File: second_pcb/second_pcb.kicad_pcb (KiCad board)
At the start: 2 copper layers, 99.2 x 69.6 mm, 194 parts, among them SW1 SW_Nidec_CAS-120A1, U1 MIC29502WU, U10 CJ432, U11 CJ432, U12 CJ432, U13 CJ432, U14 CJ432, U15 CJ432, U16 CJ432, U17 CJ432, U18 CJ432, U19 CJ432, U2 CJ432, U20 CJ432, U21 CJ432, U22 CJ432, U23 CJ432, U24 CJ432, U25 CJ432, U26 CJ432, U27 CJ432, U28 CJ432, U29 CJ432, U3 CJ432, U30 CJ432, U31 CJ432, U32 CJ432, U33 CJ432, U34 CJ432, U35 CJ432, U36 CJ432, U37 CJ432, U38 CJ432, U39 CJ432, U4 CJ432, U40 CJ432, U41 CJ432, U42 CJ432, U43 CJ432, U44 CJ432, U45 CJ432, U46 CJ432, U47 CJ432, U48 CJ432, U49 CJ432, U5 CJ432, U50 CJ432, U51 CJ432, U52 CJ432, U53 CJ432, U54 CJ432, U55 CJ432, U56 CJ432, U57 CJ432, U58 CJ432, U59 CJ432, U6 CJ432, U60 CJ432, U61 CJ432, U7 CJ432, U8 CJ432, U9 CJ432

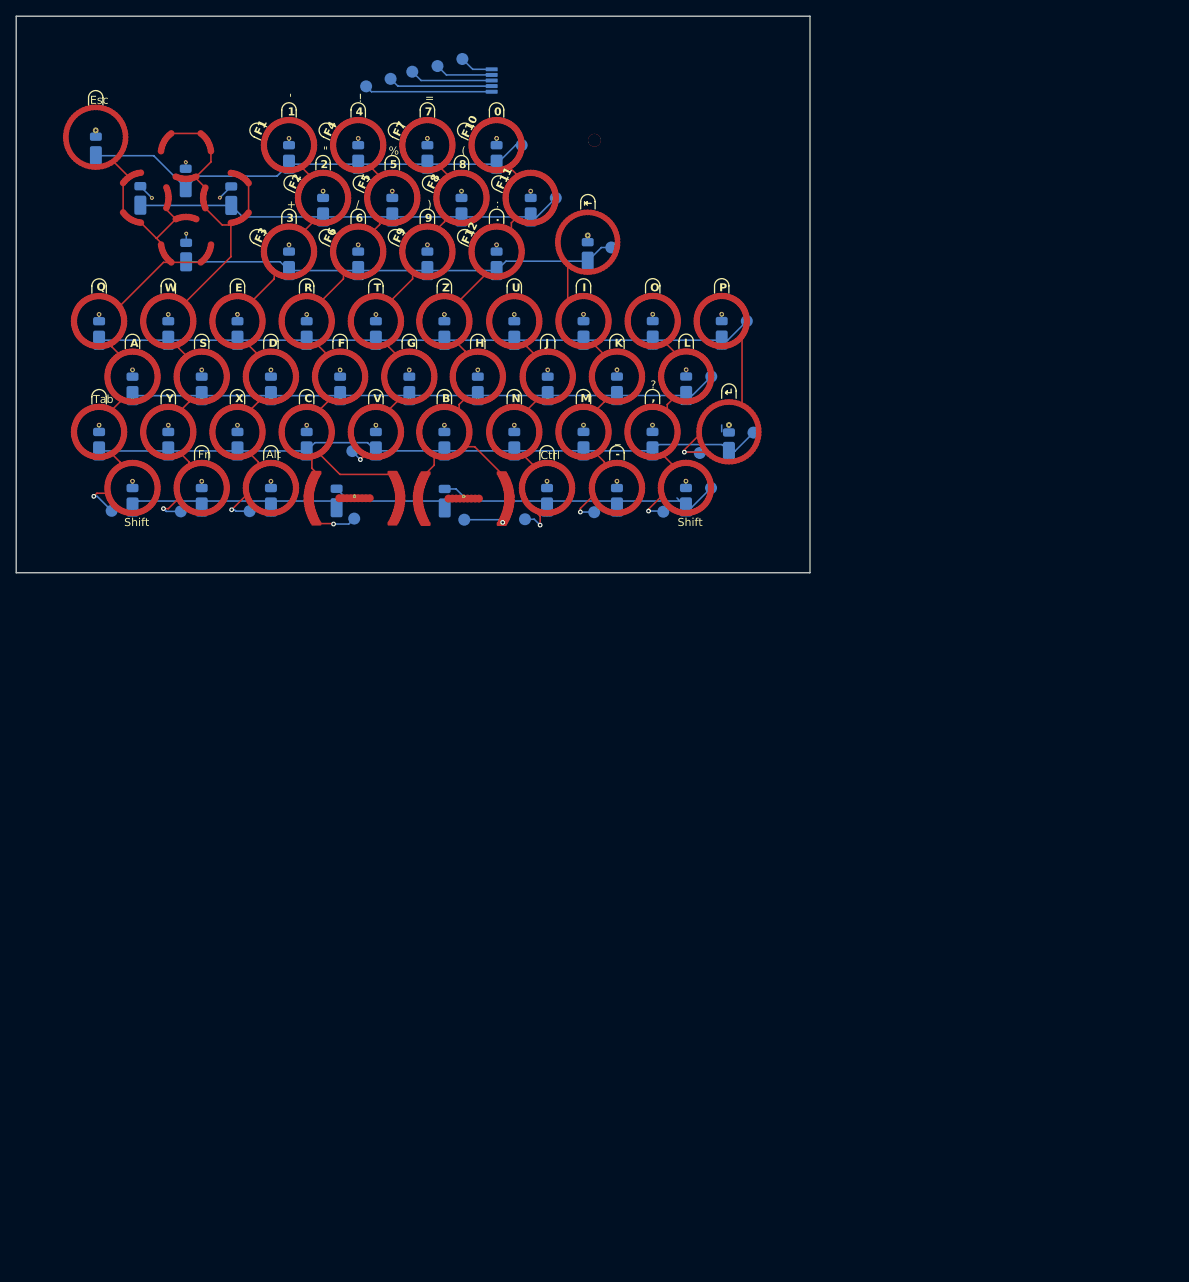
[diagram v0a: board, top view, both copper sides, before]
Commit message: full size keyboard
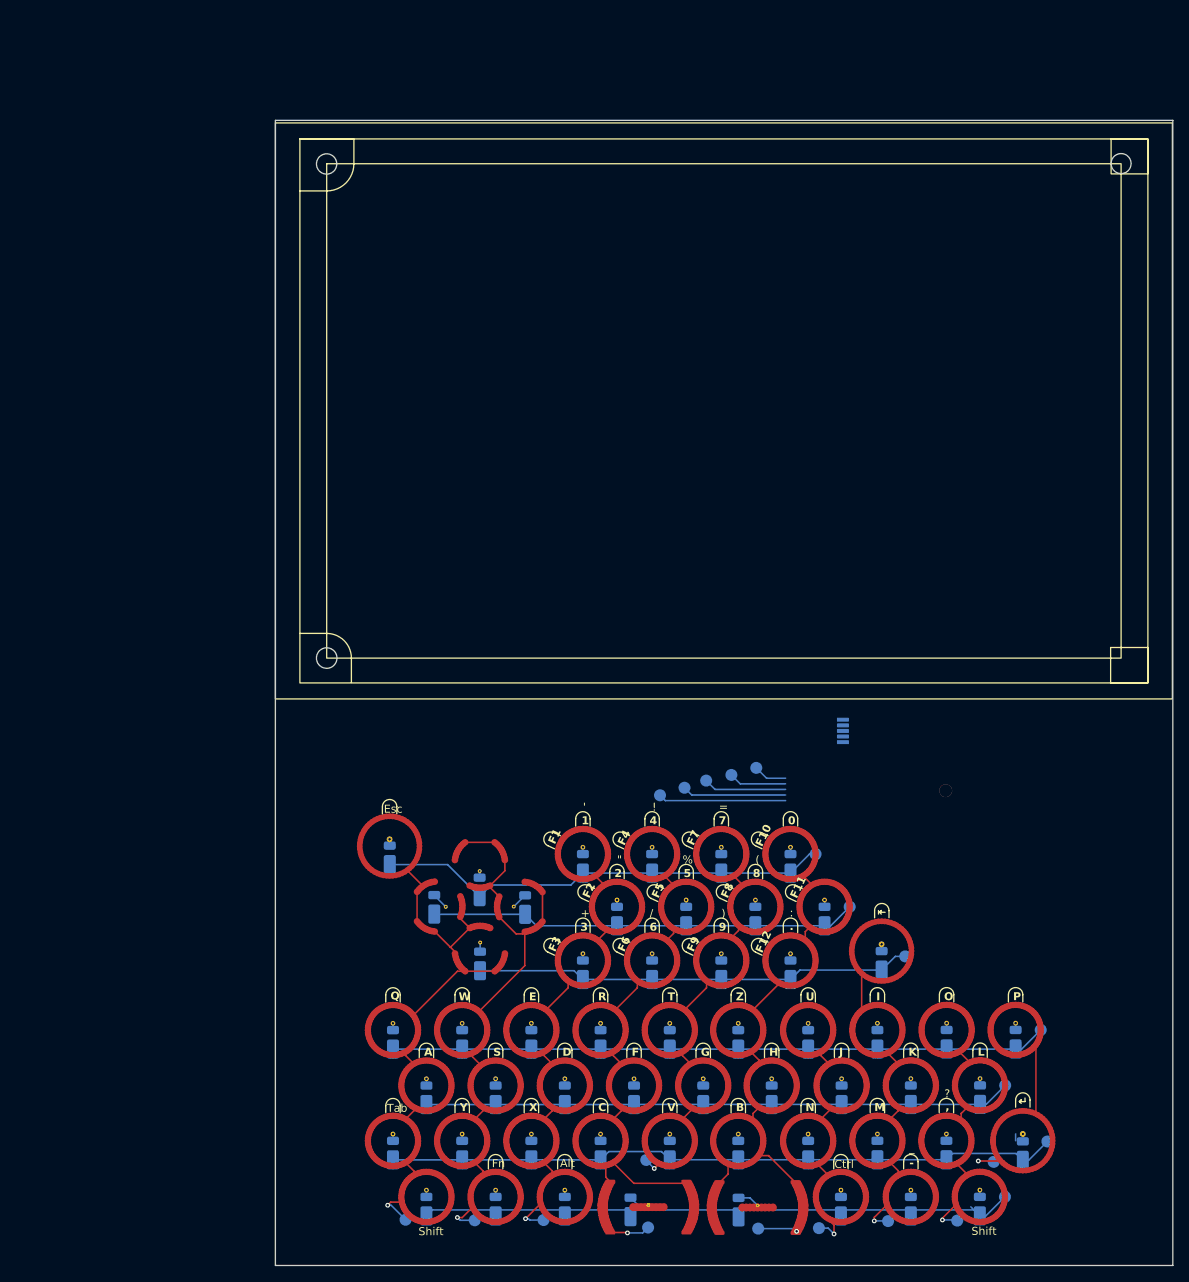
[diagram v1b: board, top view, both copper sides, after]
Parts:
- added U62: CJ432, custom_footprints:LCD, F.Cu at (108.1, 66.7)
- moved U53 96.0 mm to (70.9, 165.0)
- moved D50 95.9 mm to (96.4, 166.6)
- moved D1 95.9 mm to (66.3, 122.6)
- moved D13 95.9 mm to (77.6, 135.8)
- moved D14 95.9 mm to (90.4, 136.9)
- moved D15 95.9 mm to (99.1, 136.9)
- moved D16 95.9 mm to (107.7, 136.9)
- moved D17 95.9 mm to (116.4, 136.9)
- moved D18 95.9 mm to (66.7, 145.6)
- moved D19 95.9 mm to (75.4, 145.6)
- moved D2 95.9 mm to (77.5, 126.6)
- moved D20 95.9 mm to (84.0, 145.6)
- moved D21 95.9 mm to (92.7, 145.6)
- moved D22 95.9 mm to (101.3, 145.6)
- moved D23 95.9 mm to (109.9, 145.6)
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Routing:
- net Net-(S27-Pad1): track 18.2 -> 15.3 mm
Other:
- board size 99.2 x 69.6 mm -> 112.2 x 143.1 mm
